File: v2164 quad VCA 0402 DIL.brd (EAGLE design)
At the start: 41.3 x 16.2 mm, 45 parts, among them IC1 TL072JD, IC2 TL072JD

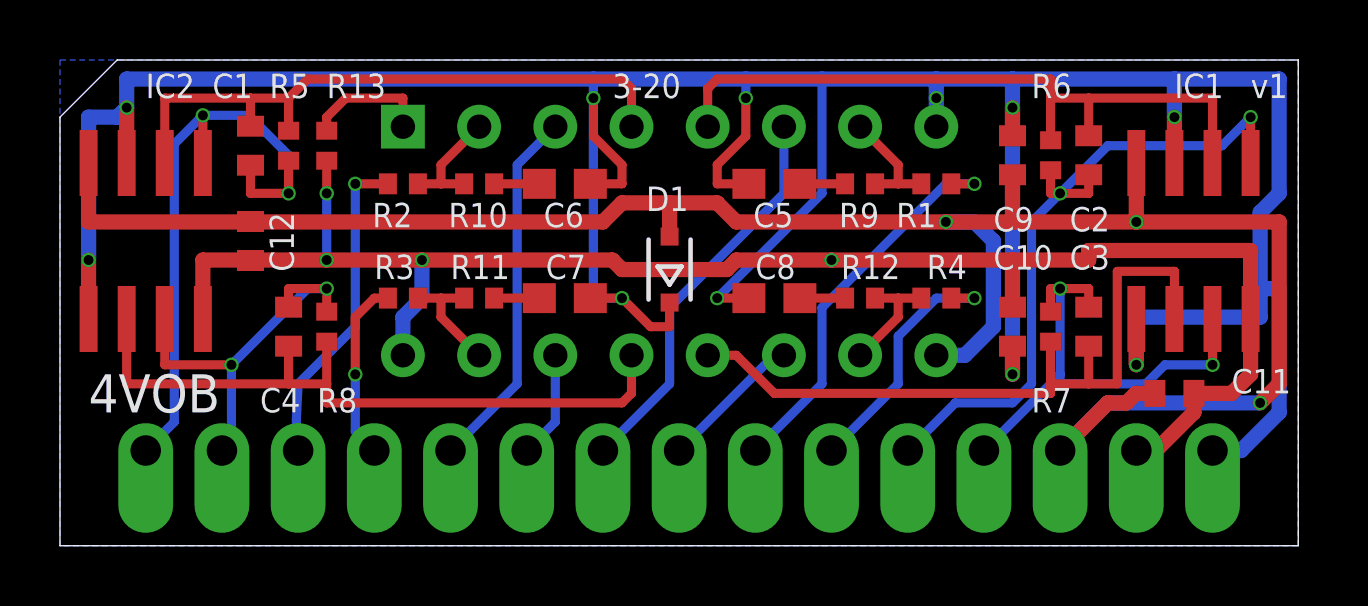
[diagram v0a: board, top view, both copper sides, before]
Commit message: Tiny placement tweak
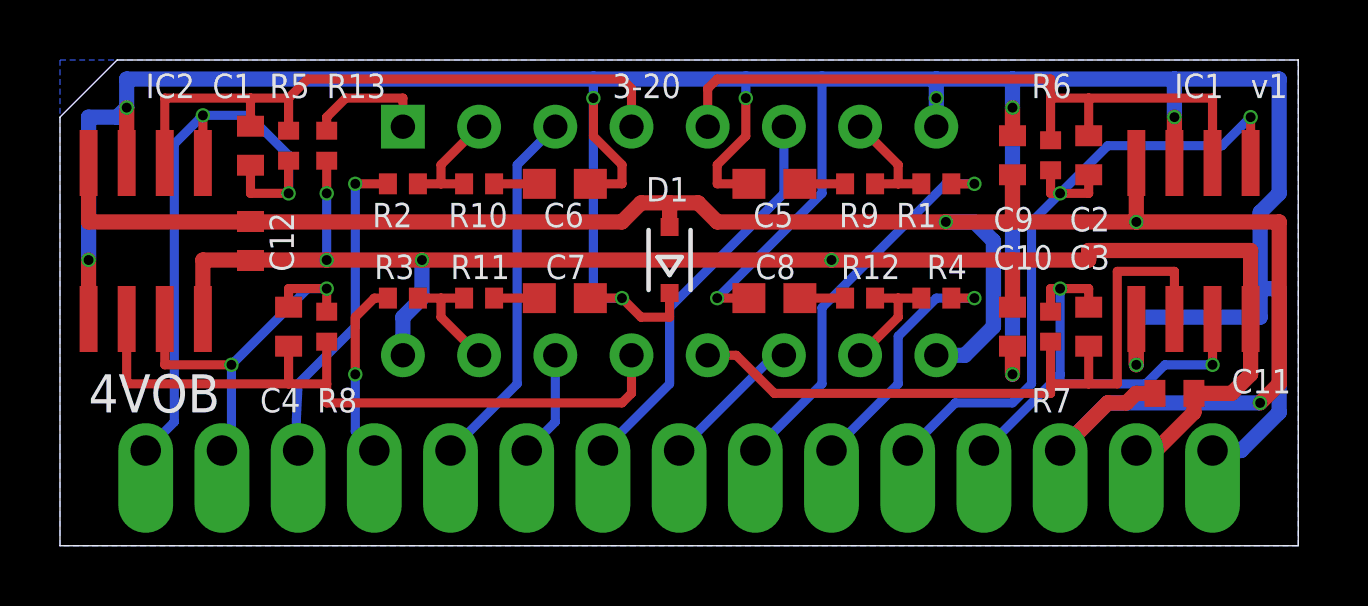
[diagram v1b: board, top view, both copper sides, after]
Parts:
- moved D1 0.32 mm to (20.3, 9.53)
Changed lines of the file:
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@@
 </element>
 <element name="U$1" library="joakim" package="XONIK_LOGO_18" value="" x="29.5275" y="8.3111" smashed="yes" rot="MR0"/>
-<element name="D1" library="diode" library_urn="urn:adsk.eagle:library:210" package="SOD323-R" package3d_urn="urn:adsk.eagle:package:43437/1" value="B5817" x="20.32" y="9.2075" smashed="yes" rot="R90">
-<attribute name="NAME" x="19.5375" y="11.16" size="0.8128" layer="25" font="vector"/>
-<attribute name="POPULARITY" value="4" x="20.32" y="9.2075" size="0.8128" layer="27" font="vector" rot="R90" display="off"/>
-<attribute name="VALUE" x="22.62" y="8.1075" size="1.27" layer="27" rot="R90"/>
+<element name="D1" library="diode" library_urn="urn:adsk.eagle:library:210" package="SOD323-R" package3d_urn="urn:adsk.eagle:package:43437/1" value="B5817" x="20.32" y="9.525" smashed="yes" rot="R90">
+<attribute name="NAME" x="19.5375" y="11.4775" size="0.8128" layer="25" font="vector"/>
+<attribute name="POPULARITY" value="4" x="20.32" y="9.525" size="0.8128" layer="27" font="vector" rot="R90" display="off"/>
+<attribute name="VALUE" x="22.62" y="8.425" size="1.27" layer="27" rot="R90"/>
 </element>
 </elements>
@@
 <wire x1="21.9075" y1="12.7" x2="22.86" y2="13.6525" width="0.3048" layer="1"/>
 <via x="22.86" y="14.9225" extent="1-16" drill="0.3302"/>
-<wire x1="18.7325" y1="8.255" x2="19.685" y2="7.3025" width="0.3048" layer="1"/>
+<wire x1="18.7325" y1="8.255" x2="19.3675" y2="7.62" width="0.3048" layer="1"/>
 <wire x1="22.86" y1="13.6525" x2="22.86" y2="14.9225" width="0.3048" layer="1"/>
 <contactref element="D1" pad="C"/>
-<wire x1="19.685" y1="7.3025" x2="20.32" y2="7.3025" width="0.3048" layer="1"/>
-<wire x1="20.32" y1="7.3025" x2="20.32" y2="8.1075" width="0.3048" layer="1"/>
+<wire x1="19.3675" y1="7.62" x2="20.32" y2="7.62" width="0.3048" layer="1"/>
+<wire x1="20.32" y1="7.62" x2="20.32" y2="8.425" width="0.3048" layer="1"/>
 </signal>
 <signal name="N$1">
@@
 <wire x1="34.29" y1="9.525" x2="31.75" y2="9.525" width="0.508" layer="1"/>
 <wire x1="31.75" y1="9.525" x2="25.7175" y2="9.525" width="0.508" layer="1"/>
-<wire x1="25.7175" y1="9.525" x2="22.5425" y2="9.525" width="0.508" layer="1"/>
-<wire x1="22.5425" y1="9.525" x2="22.225" y2="9.2075" width="0.508" layer="1"/>
-<wire x1="22.225" y1="9.2075" x2="18.7325" y2="9.2075" width="0.508" layer="1"/>
-<wire x1="18.7325" y1="9.2075" x2="18.415" y2="9.525" width="0.508" layer="1"/>
-<wire x1="18.415" y1="9.525" x2="12.065" y2="9.525" width="0.508" layer="1"/>
+<wire x1="25.7175" y1="9.525" x2="12.065" y2="9.525" width="0.508" layer="1"/>
 <wire x1="12.065" y1="9.525" x2="8.89" y2="9.525" width="0.508" layer="1"/>
 <wire x1="8.89" y1="9.525" x2="6.35" y2="9.525" width="0.508" layer="1"/>
@@
 <contactref element="C12" pad="1"/>
 <wire x1="31.75" y1="10.795" x2="29.5275" y2="10.795" width="0.508" layer="1"/>
-<wire x1="29.5275" y1="10.795" x2="22.5425" y2="10.795" width="0.508" layer="1"/>
-<wire x1="22.5425" y1="10.795" x2="21.9075" y2="11.43" width="0.508" layer="1"/>
-<wire x1="20.32" y1="11.43" x2="18.7325" y2="11.43" width="0.508" layer="1"/>
-<wire x1="18.7325" y1="11.43" x2="18.0975" y2="10.795" width="0.508" layer="1"/>
-<wire x1="18.0975" y1="10.795" x2="6.35" y2="10.795" width="0.508" layer="1"/>
+<wire x1="29.5275" y1="10.795" x2="21.9075" y2="10.795" width="0.508" layer="1"/>
+<wire x1="21.9075" y1="10.795" x2="21.2725" y2="11.43" width="0.508" layer="1"/>
+<wire x1="20.32" y1="11.43" x2="19.3675" y2="11.43" width="0.508" layer="1"/>
+<wire x1="19.3675" y1="11.43" x2="18.7325" y2="10.795" width="0.508" layer="1"/>
+<wire x1="18.7325" y1="10.795" x2="6.35" y2="10.795" width="0.508" layer="1"/>
 <wire x1="6.35" y1="10.795" x2="0.9525" y2="10.795" width="0.508" layer="1"/>
 <wire x1="29.5275" y1="10.795" x2="30.48" y2="10.795" width="0.508" layer="16"/>
@@
 <via x="35.8775" y="10.795" extent="1-16" drill="0.3302"/>
 <contactref element="D1" pad="A"/>
-<wire x1="20.32" y1="10.3075" x2="20.32" y2="11.43" width="0.508" layer="1"/>
-<wire x1="21.9075" y1="11.43" x2="20.32" y2="11.43" width="0.508" layer="1"/>
+<wire x1="20.32" y1="10.625" x2="20.32" y2="11.43" width="0.508" layer="1"/>
+<wire x1="21.2725" y1="11.43" x2="20.32" y2="11.43" width="0.508" layer="1"/>
 </signal>
 <signal name="OUT4">
